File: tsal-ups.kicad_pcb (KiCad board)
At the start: 2 copper layers, 3 parts, among them U1 TPS552892RYQR, U2 TPS2121RUXR, U3 STM32F103CBTx

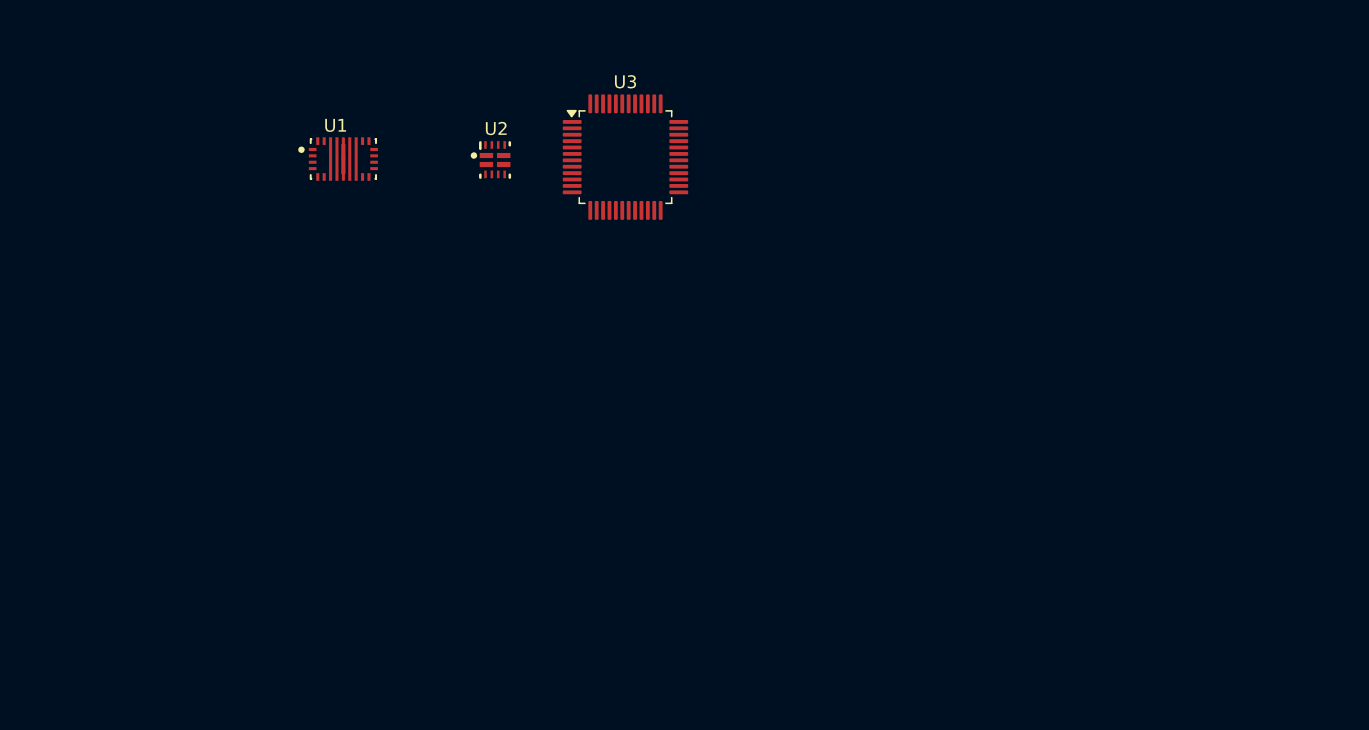
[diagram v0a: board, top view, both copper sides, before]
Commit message: Revision A
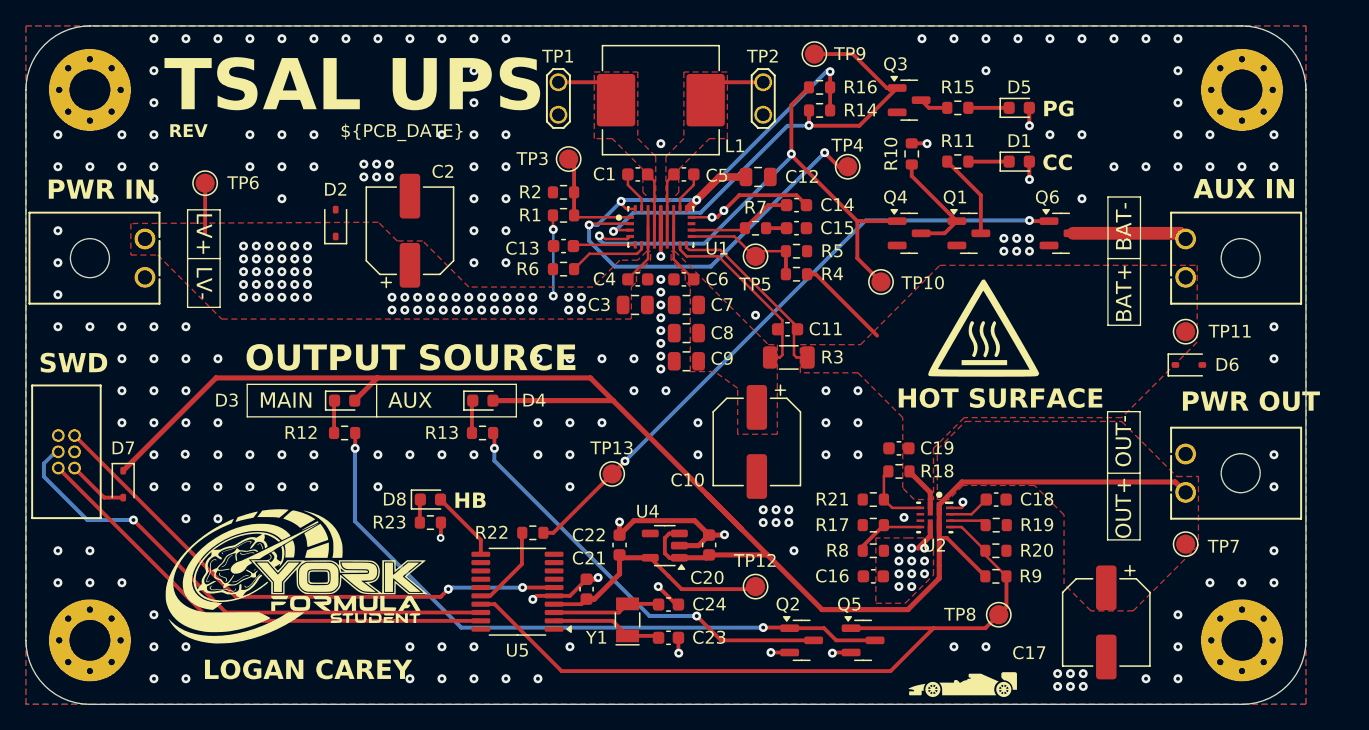
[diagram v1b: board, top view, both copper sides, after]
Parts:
- removed U3: STM32F103CBTx, Package_QFP:LQFP-48_7x7mm_P0.5mm
- added C1: 0.1u, Capacitor_SMD:C_0603_1608Metric, F.Cu at (137.8, 70.6)
- added C10: 22u, Capacitor_SMD:CP_Elec_6.3x7.7, F.Cu at (147.1, 91.5)
- added C11: 0.1u, Capacitor_SMD:C_0603_1608Metric, F.Cu at (149.5, 82.7)
- added C12: 4.7u, Capacitor_SMD:C_0805_2012Metric, F.Cu at (147.2, 70.8)
- added C13: 0.01u, Capacitor_SMD:C_0603_1608Metric, F.Cu at (132.0, 76.2)
- added C14: 56p, Capacitor_SMD:C_0603_1608Metric, F.Cu at (150.2, 73.0)
- added C15: 10n, Capacitor_SMD:C_0603_1608Metric, F.Cu at (150.2, 74.8)
- added C16: 1u, Capacitor_SMD:C_0603_1608Metric, F.Cu at (156.2, 102.0)
- added C17: 100u, Capacitor_SMD:CP_Elec_6.3x7.7, F.Cu at (174.4, 105.6)
- added C18: 0.1u, Capacitor_SMD:C_0603_1608Metric, F.Cu at (165.8, 96.0)
- added C19: 1u, Capacitor_SMD:C_0603_1608Metric, F.Cu at (158.2, 92.0)
- added C2: 22u, Capacitor_SMD:CP_Elec_6.3x7.7, F.Cu at (120.0, 75.0)
- added C20: 1u, Capacitor_SMD:C_0603_1608Metric, F.Cu at (143.4, 99.5)
- added C21: 1u, Capacitor_SMD:C_0603_1608Metric, F.Cu at (133.8, 103.0)
- added C22: 1u, Capacitor_SMD:C_0603_1608Metric, F.Cu at (136.4, 99.5)
- added C23: 20p, Capacitor_SMD:C_0603_1608Metric, F.Cu at (140.2, 106.8)
- added C24: 20p, Capacitor_SMD:C_0603_1608Metric, F.Cu at (140.2, 104.2)
- added C3: 10u, Capacitor_SMD:C_0805_2012Metric, F.Cu at (137.6, 80.8)
- added C4: 1u, Capacitor_SMD:C_0603_1608Metric, F.Cu at (137.8, 78.8)
- added C5: 0.1u, Capacitor_SMD:C_0603_1608Metric, F.Cu at (141.4, 70.6)
- added C6: 1u, Capacitor_SMD:C_0603_1608Metric, F.Cu at (141.4, 78.8)
- added C7: 4.7u, Capacitor_SMD:C_0805_2012Metric, F.Cu at (141.6, 80.8)
- added C8: 4.7u, Capacitor_SMD:C_0805_2012Metric, F.Cu at (141.6, 83.0)
- added C9: 4.7u, Capacitor_SMD:C_0805_2012Metric, F.Cu at (141.6, 85.2)
- added D1: LED, LED_SMD:LED_0603_1608Metric, F.Cu at (167.6, 69.6)
- added D2: BZX384C20, Diode_SMD:D_SOD-323, F.Cu at (114.2, 74.4)
- added D3: LED, LED_SMD:LED_0603_1608Metric, F.Cu at (114.9, 88.3)
- added D4: LED, LED_SMD:LED_0603_1608Metric, F.Cu at (125.7, 88.3)
- added D5: LED, LED_SMD:LED_0603_1608Metric, F.Cu at (167.6, 65.4)
- added D6: BZX384C20, Diode_SMD:D_SOD-323, F.Cu at (180.8, 85.5)
- added D7: D_Schottky, Diode_SMD:D_SOD-323, F.Cu at (97.6, 94.8)
- added D8: LED, LED_SMD:LED_0603_1608Metric, F.Cu at (121.6, 96.0)
- added G***: LOGO, MyLibrary:YFS Logo, F.Cu at (110.9, 102.2)
- added G***: LOGO, MyLibrary:YFS Logo, B.Cu at (167.2, 101.8)
- added G****: LOGO, LOGO, F.Cu at (164.8, 82.6)
- added G****: LOGO, LOGO, B.Cu at (164.8, 82.6)
- added H1: MountingHole_Pad, MountingHole:MountingHole_3.2mm_M3_Pad_Via, F.Cu at (95.0, 64.0)
- added H2: MountingHole_Pad, MountingHole:MountingHole_3.2mm_M3_Pad_Via, F.Cu at (185.0, 64.0)
- added H3: MountingHole_Pad, MountingHole:MountingHole_3.2mm_M3_Pad_Via, F.Cu at (185.0, 107.0)
- added H4: MountingHole_Pad, MountingHole:MountingHole_3.2mm_M3_Pad_Via, F.Cu at (95.0, 107.0)
- added J1: MAIN_IN, yfs:MolexMicrofitPlus1x2, F.Cu at (99.3, 78.6)
- added J2: AUX_IN, yfs:MolexMicrofitPlus1x2, F.Cu at (180.6, 75.6)
- added J3: VOUT, yfs:MolexMicrofitPlus1x2, F.Cu at (180.6, 92.4)
- added J4: Conn_01x06, yfs:IDC-Connector-2x3, F.Cu at (93.8, 93.5)
- added L1: 10u, Inductor_SMD:L_APV_APH0850, F.Cu at (139.6, 64.8)
- added Q1: 2N7002, Package_TO_SOT_SMD:SOT-23, F.Cu at (163.7, 75.2)
- added Q2: 2N7002, Package_TO_SOT_SMD:SOT-23, F.Cu at (150.6, 107.0)
- added Q3: 2N7002, Package_TO_SOT_SMD:SOT-23, F.Cu at (159.0, 64.8)
- added Q4: 2N7002, Package_TO_SOT_SMD:SOT-23, F.Cu at (159.0, 75.2)
- added Q5: 2N7002, Package_TO_SOT_SMD:SOT-23, F.Cu at (155.4, 107.0)
- added Q6: AO3400A, Package_TO_SOT_SMD:SOT-23, F.Cu at (170.9, 75.2)
- added R1: 383k, Resistor_SMD:R_0603_1608Metric, F.Cu at (132.0, 73.8)
- added R10: 10k, Resistor_SMD:R_0603_1608Metric, F.Cu at (159.2, 69.0)
- added R11: 1k, Resistor_SMD:R_0603_1608Metric, F.Cu at (162.8, 69.6)
- added R12: 1k, Resistor_SMD:R_0603_1608Metric, F.Cu at (114.9, 90.8)
- added R13: 1k, Resistor_SMD:R_0603_1608Metric, F.Cu at (125.7, 90.8)
- added R14: 10k, Resistor_SMD:R_0603_1608Metric, F.Cu at (152.0, 65.6)
- added R15: 1k, Resistor_SMD:R_0603_1608Metric, F.Cu at (162.8, 65.4)
- added R16: 10k, Resistor_SMD:R_0603_1608Metric, F.Cu at (152.0, 63.8)
- added R17: 3k, Resistor_SMD:R_0603_1608Metric, F.Cu at (156.2, 98.0)
- added R18: 24k, Resistor_SMD:R_0603_1608Metric, F.Cu at (158.2, 93.8)
- added R19: 21.5k, Resistor_SMD:R_0603_1608Metric, F.Cu at (165.8, 98.0)
- added R2: 100k, Resistor_SMD:R_0603_1608Metric, F.Cu at (132.0, 72.0)
- added R20: 4.3k, Resistor_SMD:R_0603_1608Metric, F.Cu at (165.8, 100.0)
- added R21: 3.3k, Resistor_SMD:R_0603_1608Metric, F.Cu at (156.2, 96.0)
- added R22: 100, Resistor_SMD:R_0603_1608Metric, F.Cu at (129.6, 98.6)
- added R23: 330, Resistor_SMD:R_0603_1608Metric, F.Cu at (121.6, 97.8)
- added R3: 25m, Resistor_SMD:R_1206_3216Metric, F.Cu at (149.6, 84.9)
- added R4: 100k, Resistor_SMD:R_0603_1608Metric, F.Cu at (150.2, 78.4)
- added R5: 9.76k, Resistor_SMD:R_0603_1608Metric, F.Cu at (150.2, 76.6)
- added R6: 48.7k, Resistor_SMD:R_0603_1608Metric, F.Cu at (132.0, 78.0)
- added R7: 9.09k, Resistor_SMD:R_0603_1608Metric, F.Cu at (147.0, 74.8)
- added R8: 18k, Resistor_SMD:R_0603_1608Metric, F.Cu at (156.2, 100.0)
- added R9: 15k, Resistor_SMD:R_0603_1608Metric, F.Cu at (165.8, 102.0)
- added TP1: TestPoint_2Pole, yfs:TestPoint_2Pads_Pitch2.54mm_Drill1.0mm, F.Cu at (131.6, 63.4)
- added TP10: TestPoint, TestPoint:TestPoint_Pad_D1.5mm, F.Cu at (156.8, 79.0)
- added TP11: TestPoint, TestPoint:TestPoint_Pad_D1.5mm, F.Cu at (180.6, 82.9)
- added TP12: TestPoint, TestPoint:TestPoint_Pad_D1.5mm, F.Cu at (147.0, 102.8)
- added TP13: TestPoint, TestPoint:TestPoint_Pad_D1.5mm, F.Cu at (135.8, 94.0)
- added TP2: TestPoint_2Pole, yfs:TestPoint_2Pads_Pitch2.54mm_Drill1.0mm, F.Cu at (147.6, 63.4)
- added TP3: TestPoint, TestPoint:TestPoint_Pad_D1.5mm, F.Cu at (132.4, 69.4)
- added TP4: TestPoint, TestPoint:TestPoint_Pad_D1.5mm, F.Cu at (154.2, 70.0)
- added TP5: TestPoint, TestPoint:TestPoint_Pad_D1.5mm, F.Cu at (147.0, 77.0)
- added TP6: TestPoint, TestPoint:TestPoint_Pad_D1.5mm, F.Cu at (104.0, 71.3)
- added TP7: TestPoint, TestPoint:TestPoint_Pad_D1.5mm, F.Cu at (180.6, 99.5)
- added TP8: TestPoint, TestPoint:TestPoint_Pad_D1.5mm, F.Cu at (166.0, 105.0)
- added TP9: TestPoint, TestPoint:TestPoint_Pad_D1.5mm, F.Cu at (151.6, 61.2)
- added U4: AP7383, Package_TO_SOT_SMD:TSOT-23-5, F.Cu at (139.9, 99.6)
- added U5: STM32C011F4Px, Package_SO:TSSOP-20_4.4x6.5mm_P0.65mm, F.Cu at (128.4, 103.2)
- added Y1: 32.768k, Crystal:Crystal_SMD_G8-2Pin_3.2x1.5mm, F.Cu at (137.0, 105.4)
- moved U2 44.3 mm to (161.0, 97.4), turned to -90 degrees
- moved U1 25.4 mm to (139.6, 74.7)
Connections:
- U1 pad 1: unconnected-(U1-EN_UVLO-Pad1) -> /EN/UVLO
- U1 pad 10: unconnected-(U1-SW2-Pad10) -> /SW2
- U1 pad 11: unconnected-(U1-VOUT-Pad11) -> /ISP
- U1 pad 12: unconnected-(U1-ISP-Pad12) -> /ISP
- U1 pad 13: unconnected-(U1-ISN-Pad13) -> +12V_AUX
- U1 pad 14: unconnected-(U1-FB-Pad14) -> /FB
- U1 pad 15: unconnected-(U1-COMP-Pad15) -> /COMP
- U1 pad 17: unconnected-(U1-AGND-Pad17) -> GND
- U1 pad 18: unconnected-(U1-VCC-Pad18) -> +5V_INT
- U1 pad 19: unconnected-(U1-BOOT2-Pad19) -> Net-(U1-BOOT2)
- U1 pad 2: unconnected-(U1-MODE-Pad2) -> +5V_INT
- U1 pad 20: unconnected-(U1-BOOT1-Pad20) -> Net-(U1-BOOT1)
- U1 pad 21: unconnected-(U1-EXTVCC-Pad21) -> +5V_INT
- U1 pad 3: unconnected-(U1-PG-Pad3) -> /PG
- U1 pad 4: unconnected-(U1-~{CC}-Pad4) -> /~{CC}
- U1 pad 5: unconnected-(U1-DITH_SYNC-Pad5) -> /DITH_SYNC
- U1 pad 6: unconnected-(U1-FSW-Pad6) -> /FSW
- U1 pad 7: unconnected-(U1-VIN-Pad7) -> +12V_MAIN
- U1 pad 8: unconnected-(U1-SW1-Pad8) -> /SW1
- U1 pad 9: unconnected-(U1-PGND-Pad9) -> GND
- U2 pad 1: unconnected-(U2-OUT-Pad1) -> +12V_OUT
- U2 pad 10: unconnected-(U2-ILM-Pad10) -> /I_LIMIT
- U2 pad 11: unconnected-(U2-SS-Pad11) -> /SOFT_START
- U2 pad 12: unconnected-(U2-GND-Pad12) -> GND
- U2 pad 2: unconnected-(U2-IN2-Pad2) -> +12V_AUX
- U2 pad 3: unconnected-(U2-CP2-Pad3) -> /CP2
- U2 pad 4: unconnected-(U2-OV2-Pad4) -> GND
- U2 pad 5: unconnected-(U2-OV1-Pad5) -> GND
- U2 pad 6: unconnected-(U2-PR1-Pad6) -> /PR1
- U2 pad 7: unconnected-(U2-IN1-Pad7) -> +12V_MAIN
- U2 pad 8: unconnected-(U2-OUT-Pad8) -> +12V_OUT
- U2 pad 9: unconnected-(U2-ST-Pad9) -> STATUS
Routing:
- net +12V_OUT: track 0.00 -> 134.8 mm
- net +5V_INT: track 0.00 -> 63.4 mm, vias 0 -> 5
- net STATUS: track 0.00 -> 60.4 mm
- net Net-(Q2-G): track 0.00 -> 51.1 mm, vias 0 -> 2
- net Net-(Q6-G): track 0.00 -> 49.7 mm, vias 0 -> 2
- net /Microcontroller/NRST: track 0.00 -> 43.3 mm, vias 0 -> 2
- net /~{CC}: track 0.00 -> 42.8 mm, vias 0 -> 2
- net /Microcontroller/SWDIO: track 0.00 -> 41.1 mm, vias 0 -> 1
- net GND: track 0.00 -> 39.9 mm, vias 0 -> 208
- net /Microcontroller/SWCLK: track 0.00 -> 38.0 mm
- net /PG: track 0.00 -> 37.0 mm, vias 0 -> 2
- net Net-(Q2-D): track 0.00 -> 32.7 mm, vias 0 -> 2
- net +12V_AUX: track 0.00 -> 25.7 mm
- net +12V_MAIN: track 0.00 -> 21.1 mm, vias 0 -> 74
- net +3.3V: track 0.00 -> 19.4 mm
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- added copper zone on F.Cu, net +12V_AUX
- added copper zone on F.Cu, net +12V_MAIN
- added copper zone on In2.Cu, net +12V_MAIN
- added copper zone on F.Cu, net +12V_OUT
- added copper zone on F.Cu, net /ISP
- added copper zone on F.Cu, net /SW1
- added copper zone on F.Cu, net /SW2
- added copper zone on B.Cu, net GND
- added copper zone on F.Cu, net GND
- added copper zone on In1.Cu, net GND
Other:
- board outline added: 100 x 53 mm
- copper layers 2 -> 4
- board text added: "${PCB_DATE}"
- board text added: "AUX"
- board text added: "AUX IN"
- board text added: "BAT+"
- board text added: "BAT-"
- board text added: "CC"
- board text added: "HB"
- board text added: "HOT SURFACE"
- board text added: "LOGAN CAREY"
- board text added: "LV+"
- board text added: "LV-"
- board text added: "MAIN"
- board text added: "OUT+"
- board text added: "OUT-"
- board text added: "OUTPUT SOURCE"
- board text added: "PG"
- board text added: "PWR IN"
- board text added: "PWR OUT"
- board text added: "REV ${REVISION}"
- board text added: "SWD"
- board text added: "TSAL UPS"
- board text added: "{ "ViaStitching": "0.2", "stitch_zone_0": { "HSpacing": "1", "VSpacing": "1", "HOffset": "0", "VOffset": "0", "Clearance": "0", "Randomize": false } }"
- board text added: "{ "ViaStitching": "0.2", "stitch_zone_0": { "HSpacing": "1", "VSpacing": "1", "HOffset": "0", "VOffset": "0", "Clearance": "1", "Randomize": false } }"
